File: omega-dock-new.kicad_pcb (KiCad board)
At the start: 2 copper layers, 43 x 40 mm, 19 parts, among them J1 USB_A, J2 Conn_01x02, J3 RJ45-TRAFO, U1 USBLC6-2, U2 AP111733, U3 OMEGA_2

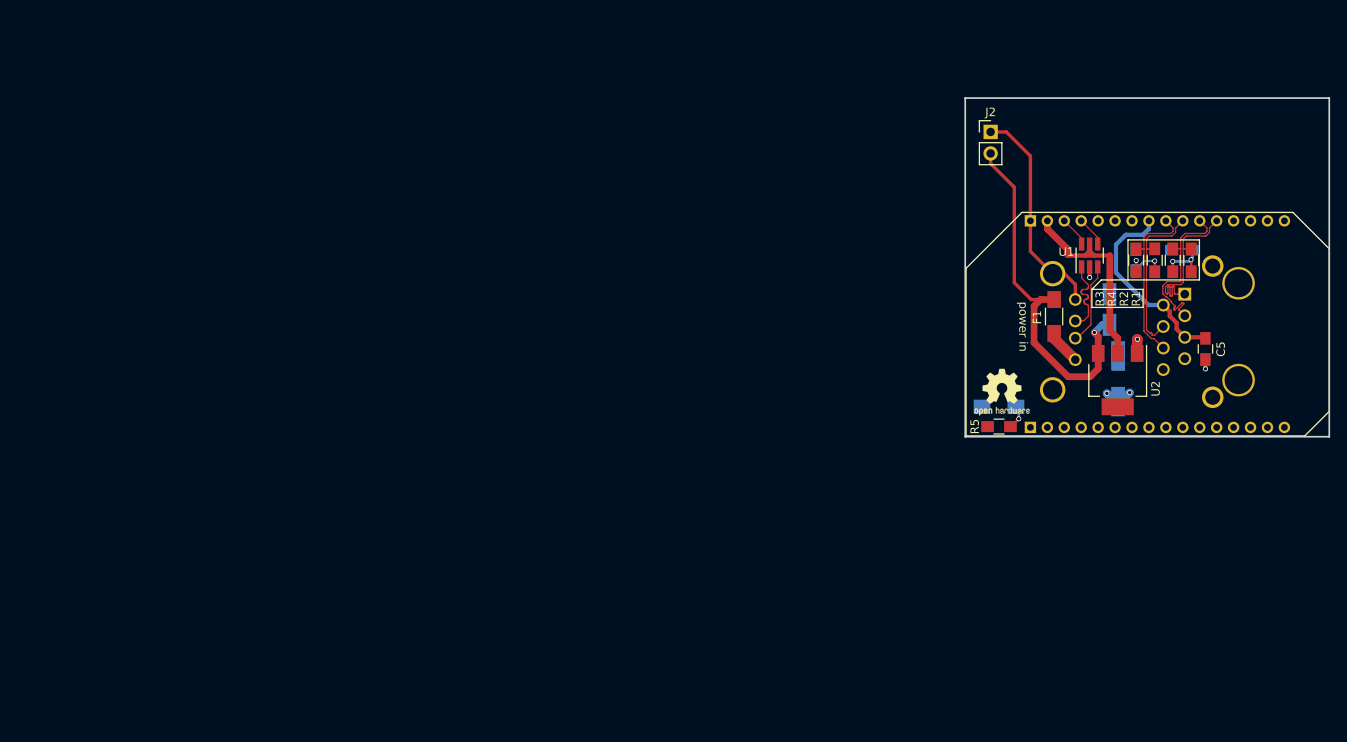
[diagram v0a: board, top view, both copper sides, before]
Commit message: actualizando todos los perifericos
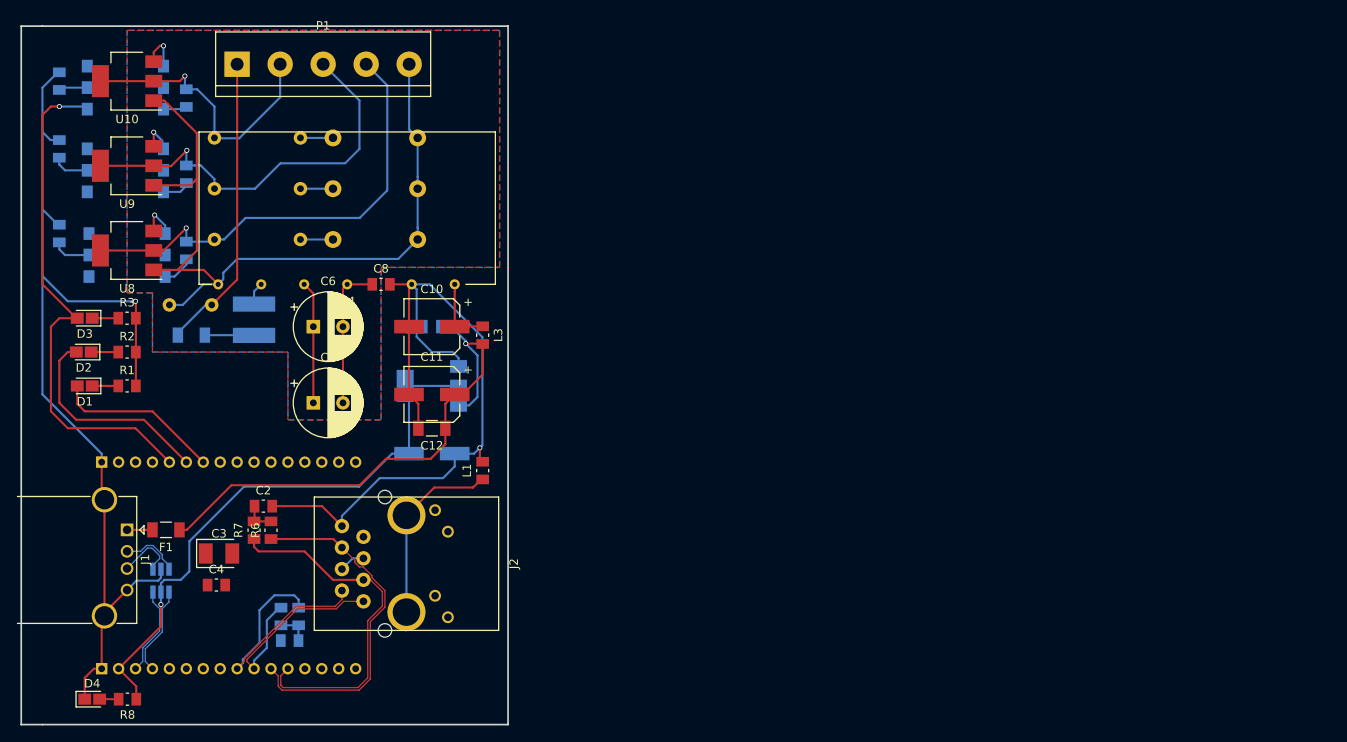
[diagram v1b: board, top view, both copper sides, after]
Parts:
- removed J3: RJ45-TRAFO, RJ45-TRAFO-AMPHENOL:RJ45_TRAFO_AMPHENOL
- removed REF***: OSHW-Logo2_7.3x6mm_SilkScreen, Symbols:OSHW-Logo2_7.3x6mm_SilkScreen
- added C10: 270uF, Capacitor_SMD:CP_Elec_6.3x7.7, F.Cu at (91.0, 58.0)
- added C11: 68uF, Capacitor_SMD:CP_Elec_6.3x7.7, F.Cu at (91.0, 66.0)
- added C12: 100nF, Capacitor_SMD:C_1206_3216Metric_Pad1.24x1.80mm_HandSolder, F.Cu at (91.0, 70.0)
- added C13: 1nF, Capacitor_THT:C_Rect_L13.0mm_W4.0mm_P10.00mm_FKS3_FKP3_MKS4, B.Cu at (79.3, 47.7)
- added C14: 1nF, Capacitor_THT:C_Rect_L13.0mm_W4.0mm_P10.00mm_FKS3_FKP3_MKS4, B.Cu at (79.3, 41.7)
- added C15: 1nF, Capacitor_THT:C_Rect_L13.0mm_W4.0mm_P10.00mm_FKS3_FKP3_MKS4, B.Cu at (79.3, 35.7)
- added C6: 4,7uF, Capacitor_THT:CP_Radial_D8.0mm_P3.50mm, F.Cu at (77.0, 58.0)
- added C7: 10uF, Capacitor_SMD:CP_Elec_4x5.3, B.Cu at (91.0, 58.0)
- added C8: 1nF, Capacitor_SMD:C_0805_2012Metric_Pad1.15x1.50mm_HandSolder, F.Cu at (85.0, 53.0)
- added C9: 100uF, Capacitor_SMD:CP_Elec_6.3x5.3, B.Cu at (91.0, 73.0)
- added D2: LED, LED_SMD:LED_0805_2012Metric_Castellated, F.Cu at (49.9, 61.0)
- added D3: LED, LED_SMD:LED_0805_2012Metric_Castellated, F.Cu at (50.0, 57.0)
- added D4: PWR, LED_SMD:LED_0805_2012Metric_Castellated, F.Cu at (50.9, 102.0)
- added L1: 220@100MHz, Inductor_SMD:L_0805_2012Metric_Pad1.15x1.50mm_HandSolder, F.Cu at (97.0, 75.0)
- added L2: SDR0503-472JL, Devices_MSS:SDR0503-XXX, B.Cu at (70.0, 57.2)
- added L3: 74479776247, Inductor_SMD:L_0805_2012Metric_Pad1.15x1.50mm_HandSolder, F.Cu at (97.0, 59.0)
- added P1: POWER I/O, TerminalBlock:TerminalBlock_bornier-5_P5.08mm, F.Cu at (68.0, 27.0)
- added R10: 330, Resistor_SMD:R_0805_2012Metric_Pad1.15x1.50mm_HandSolder, B.Cu at (47.0, 47.0)
- added R11: 330, Resistor_SMD:R_0805_2012Metric_Pad1.15x1.50mm_HandSolder, B.Cu at (47.0, 37.0)
- added R12: 330, Resistor_SMD:R_0805_2012Metric_Pad1.15x1.50mm_HandSolder, B.Cu at (47.0, 29.0)
- added R13: 330, Resistor_SMD:R_0805_2012Metric_Pad1.15x1.50mm_HandSolder, B.Cu at (62.0, 49.0)
- added R14: 330, Resistor_SMD:R_0805_2012Metric_Pad1.15x1.50mm_HandSolder, B.Cu at (62.0, 40.0)
- added R15: 330, Resistor_SMD:R_0805_2012Metric_Pad1.15x1.50mm_HandSolder, B.Cu at (62.0, 31.0)
- added R16: 33, Resistor_THT:R_Axial_DIN0207_L6.3mm_D2.5mm_P10.16mm_Horizontal, B.Cu at (65.3, 47.7)
- added R17: 100, Resistor_THT:R_Axial_DIN0207_L6.3mm_D2.5mm_P10.16mm_Horizontal, B.Cu at (65.3, 41.7)
- added R18: 33, Resistor_THT:R_Axial_DIN0207_L6.3mm_D2.5mm_P10.16mm_Horizontal, B.Cu at (65.3, 35.7)
- added R6: 50R, Resistor_SMD:R_0805_2012Metric_Pad1.15x1.50mm_HandSolder, F.Cu at (72.0, 82.0)
- added R7: 50R, Resistor_SMD:R_0805_2012Metric_Pad1.15x1.50mm_HandSolder, F.Cu at (70.0, 82.0)
- added R8: 150R, Resistor_SMD:R_0805_2012Metric_Pad1.15x1.50mm_HandSolder, F.Cu at (55.0, 102.0)
- added R9: 300k, Resistor_SMD:R_1206_3216Metric_Pad1.24x1.80mm_HandSolder, B.Cu at (62.6, 59.0)
- added RV1: B72214S0351K101, Capacitor_THT:C_Disc_D4.3mm_W1.9mm_P5.00mm, B.Cu at (65.0, 55.4)
- added U10: Z0103MN 5AA4, Devices_MSS:SOT-223-Z01, F.Cu at (55.0, 29.0)
- added U4: PBO-3-S5, Devices_MSS:PBO-3-S5, F.Cu at (81.0, 53.0)
- added U5: MOC3063S-TA1, Devices_MSS:MOC306X, B.Cu at (55.0, 49.5)
- added U6: MOC3063S-TA1, Devices_MSS:MOC306X, B.Cu at (54.8, 39.5)
- added U7: MOC3063S-TA1, Devices_MSS:MOC306X, B.Cu at (54.8, 29.8)
- added U8: Z0103MN 5AA4, Devices_MSS:SOT-223-Z01, F.Cu at (55.0, 49.0)
- added U9: Z0103MN 5AA4, Devices_MSS:SOT-223-Z01, F.Cu at (55.0, 39.0)
- C1: value 10uF -> 100nF; footprint Capacitors_SMD:CP_Elec_4x5.3 -> Capacitor_SMD:C_0805_2012Metric_Pad1.15x1.50mm_HandSolder
- C2: value 100uF -> 100nF; footprint Capacitors_SMD:CP_Elec_6.3x5.3 -> Capacitor_SMD:C_0805_2012Metric_Pad1.15x1.50mm_HandSolder; moved to F.Cu
- C3: value 100nF -> 47uF; footprint Capacitors_SMD:C_0805_HandSoldering -> Capacitor_Tantalum_SMD:CP_EIA-3528-12_Kemet-T_Pad1.63x2.40mm_HandSolder; moved to F.Cu
- C4: value 100nF -> 1nF; footprint Capacitors_SMD:C_0805_HandSoldering -> Capacitor_SMD:C_0805_2012Metric_Pad1.15x1.50mm_HandSolder; moved to F.Cu
- C5: value 1uF -> 4,7uF; footprint Capacitors_SMD:C_0805_HandSoldering -> Capacitor_THT:CP_Radial_D8.0mm_P3.50mm
- D1: value PWR -> LED; footprint LEDs:LED_1206_HandSoldering -> LED_SMD:LED_0805_2012Metric_Castellated; moved to F.Cu
- F1: footprint Capacitors_SMD:C_1206_HandSoldering -> Capacitor_SMD:C_1206_3216Metric_Pad1.24x1.80mm_HandSolder
- J1: footprint Connectors:USB_A -> Connector_USB:USB_A_Horizontal; moved to F.Cu
- J2: value Conn_01x02 -> RJMG1BD3B8K1ANR; footprint Connector_PinHeader_2.54mm:PinHeader_1x02_P2.54mm_Vertical -> Devices_MSS:RJMG1B
- R1, R2, R3: value 50R -> 220; footprint Resistors_SMD:R_0805_HandSoldering -> Resistor_SMD:R_0805_2012Metric_Pad1.15x1.50mm_HandSolder
- R4: footprint Resistors_SMD:R_0805_HandSoldering -> Resistor_SMD:R_0805_2012Metric_Pad1.15x1.50mm_HandSolder; moved to B.Cu
- R5: value 150R -> 50R; footprint Resistors_SMD:R_0805_HandSoldering -> Resistor_SMD:R_0805_2012Metric_Pad1.15x1.50mm_HandSolder; moved to B.Cu
- U1: footprint TO_SOT_Packages_SMD:SOT-23-6_Handsoldering -> Package_TO_SOT_SMD:SOT-23-6_Handsoldering; moved to B.Cu
- U2: value AP111733 -> OMEGA_2; footprint TO_SOT_Packages_SMD:SOT-223 -> Devices_MSS:OMEGA_2; moved to B.Cu
- U3: value OMEGA_2 -> AP111733; footprint omega:Socket_Strip_Straight_1x16_Pitch2.00mm -> Package_TO_SOT_SMD:SOT-223; moved to B.Cu
- moved R1 126.6 mm to (55.0, 65.0), turned to 0 degrees
- moved R2 124.0 mm to (55.0, 61.0), turned to 0 degrees
- moved U2 120.4 mm to (52.0, 74.0)
- moved R3 119.4 mm to (55.0, 57.0), turned to 0 degrees
- moved C3 119.3 mm to (65.9, 84.8)
- moved U1 116.2 mm to (59.0, 88.0), turned to 270 degrees
- moved C4 115.2 mm to (65.5, 88.5), turned to 0 degrees
- moved J1 113.8 mm to (55.0, 82.0), turned to 270 degrees
- moved R4 109.5 mm to (75.3, 92.2), turned to 90 degrees
- moved D1 108.0 mm to (50.0, 65.0), turned to 180 degrees
- moved F1 107.9 mm to (59.6, 82.0), turned to 180 degrees
- moved C5 105.6 mm to (77.0, 67.0), turned to 0 degrees
- moved C1 104.4 mm to (74.2, 95.1), turned to 0 degrees
- moved C2 102.1 mm to (71.1, 79.2), turned to 0 degrees
- moved R5 87.7 mm to (73.2, 92.2), turned to 90 degrees
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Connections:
- C1 pad 1: +5V -> GND
- C1 pad 2: GND -> Net-(C1-Pad2)
- C2 pad 1: +3V3 -> Net-(C2-Pad1)
- C3 pad 1: GND -> ETH_PWR
- C3 pad 2: Net-(C3-Pad2) -> GND
- C4 pad 1: Net-(C4-Pad1) -> ETH_PWR
- C5 pad 1: ETH_PWR -> Net-(C5-Pad1)
- C5 pad 2: GND -> Net-(C5-Pad2)
- D1 pad 1: GND -> Net-(D1-Pad1)
- D1 pad 2: Net-(D1-Pad2) -> /OutTriac/Resistencia
- J2 pad 1: GND -> /TX+
- J2 pad 2: +5V -> /TX-
- R1 pad 1: Net-(C3-Pad2) -> Net-(D1-Pad1)
- R1 pad 2: /RX+ -> GND
- R2 pad 1: Net-(C3-Pad2) -> Net-(D2-Pad1)
- R2 pad 2: /RX- -> GND
- R3 pad 1: /TX- -> Net-(D3-Pad1)
- R3 pad 2: Net-(C4-Pad1) -> GND
- R4 pad 1: /TX+ -> Net-(C1-Pad2)
- R4 pad 2: Net-(C4-Pad1) -> /TX-
- R5 pad 1: +3V3 -> Net-(C1-Pad2)
- R5 pad 2: Net-(D1-Pad2) -> /TX+
- U2 pad 2: +3V3 -> (no net)
- U2 pad 3: +5V -> (no net)
- U2 pad 4: +3V3 -> (no net)
- U3 pad 2: (no net) -> +3V3
- U3 pad 3: (no net) -> +5V
- U3 pad 4: (no net) -> +3V3
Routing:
- net GND: track 29.9 -> 207.1 mm, vias 3 -> 2
- net Nac: track 0.00 -> 94.4 mm
- net /OutTriac/Compresor: track 0.00 -> 61.6 mm, vias 0 -> 1
- net VE: track 0.00 -> 55.0 mm, vias 0 -> 1
- net RE: track 0.00 -> 48.8 mm, vias 0 -> 1
- net +3V3: track 27.9 -> 68.8 mm, vias 2 -> 1
- net Vac: track 0.00 -> 35.3 mm
- net CO: track 0.00 -> 33.4 mm, vias 0 -> 1
- net /OutTriac/Ventilador: track 0.00 -> 25.3 mm
- net GNDREF: track 0.00 -> 22.2 mm
- net /RX+: track 20.7 -> 42.3 mm
- net +5V: track 43.6 -> 64.6 mm
- net ETH_PWR: track 23.4 -> 3.07 mm
- net /RX-: track 21.5 -> 41.4 mm
- net /OutTriac/Resistencia: track 0.00 -> 19.8 mm
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- added copper zone on B.Cu, net Nac
- added copper zone on F.Cu, net Nac
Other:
- board size 43 x 40 mm -> 57.5 x 82.5 mm
- board text removed: "dock\new"
- board text removed: "ethernet"
- board text removed: "omega2/2+"
- board text removed: "power in"
- board text removed: "usb host"
